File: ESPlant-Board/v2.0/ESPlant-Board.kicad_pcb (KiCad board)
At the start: 2 copper layers, 24 x 181.8 mm, 31 parts, among them J1 Conn_02x04_Counter_Clockwise, U1 ESP32-S2-MINI-1-N4, U2 BH-AAA-B5AK001, U3 Reset, U4 Boot, U5 Temp/Humid-Sensor, U6 Light sensor, U7 AMS1117-3_3, U8 MK-12C02-G025

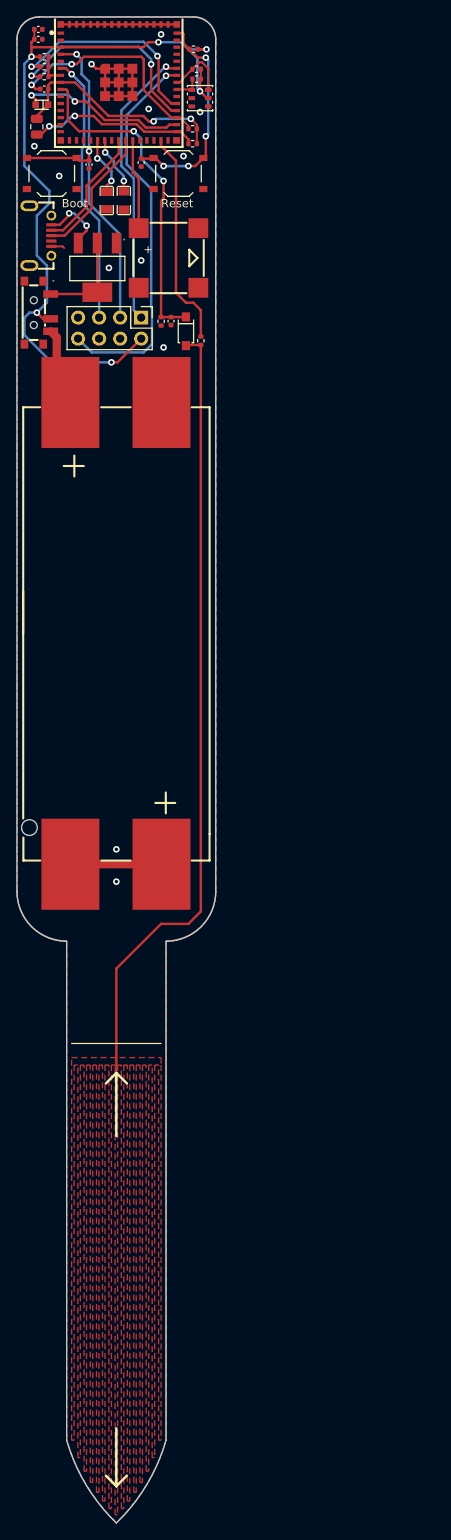
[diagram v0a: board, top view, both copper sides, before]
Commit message: Board: Update panel
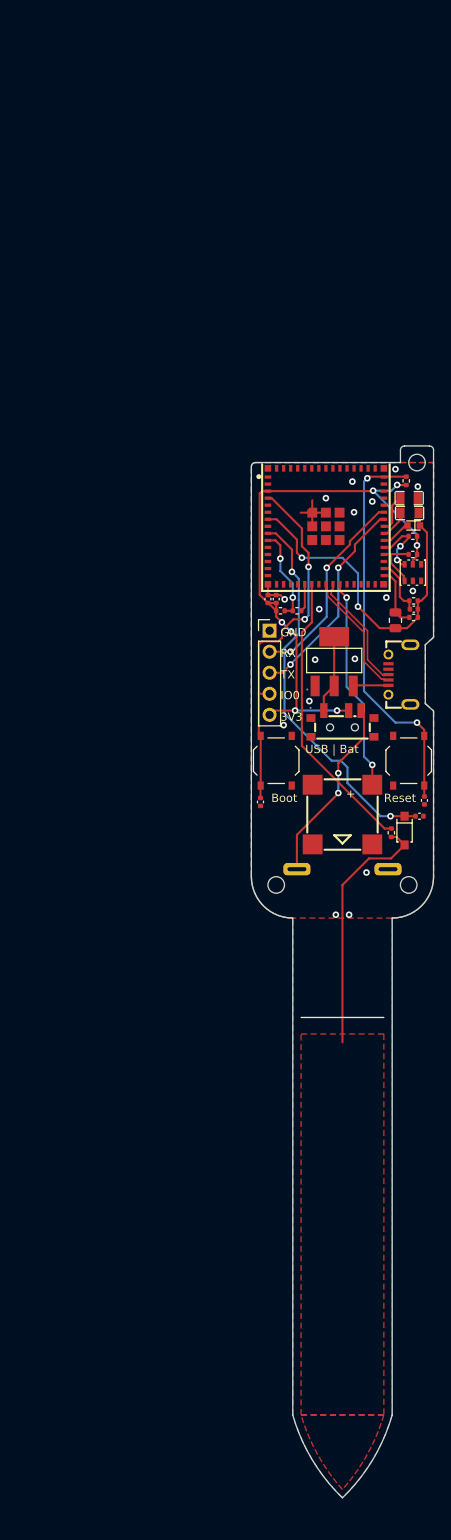
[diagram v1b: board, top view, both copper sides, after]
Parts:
- removed R5: 10k, Resistor_SMD:R_0402_1005Metric
- removed R7: 1M, Resistor_SMD:R_0402_1005Metric
- removed U2: BH-AAA-B5AK001, CustomFootprints:BAT-SMD_BH-AAA-B5AA001
- added U9: ~, CustomFootprints:AAA Battery-spring, B.Cu at (248.5, 149.1)
- C3: value 1uF -> 150pF
- J1: value Conn_02x04_Counter_Clockwise -> Conn_01x05; footprint Connector_PinHeader_2.54mm:PinHeader_2x04_P2.54mm_Vertical -> Connector_PinHeader_2.54mm:PinHeader_1x05_P2.54mm_Vertical
- moved C1 84.3 mm to (258.4, 140.8)
- moved C2 79.7 mm to (238.6, 141.0)
- moved C5 77.0 mm to (257.2, 117.7)
- moved U3 76.2 mm to (256.5, 136.0), turned to 90 degrees
- moved U4 75.9 mm to (240.5, 136.0), turned to -90 degrees
- moved C8 74.5 mm to (240.5, 116.5), turned to 90 degrees
- moved C7 73.7 mm to (254.9, 119.0), turned to 90 degrees
- moved C9 73.0 mm to (239.5, 116.5), turned to 90 degrees
- moved R4 72.7 mm to (241.1, 117.9)
- moved R6 71.4 mm to (243.1, 117.9), turned to 0 degrees
- moved BZ1 70.4 mm to (248.5, 142.5), turned to 180 degrees
- moved USB1 68.5 mm to (255.4, 125.6), turned to 90 degrees
- moved U6 67.8 mm to (257.1, 107.6)
- moved C3 66.9 mm to (257.8, 142.7), turned to 180 degrees
- moved D2 65.8 mm to (256.0, 144.4)
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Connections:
- J1 pad 1: /RX -> GND
- J1 pad 2: +3V3 -> /RX
- J1 pad 3: /IO0 -> /TX
- J1 pad 4: unconnected-(J1-Pin_4-Pad4) -> /IO0
- J1 pad 5: /IO2 -> +3V3
- R6 pad 2: /Voltage_Measurement_Select_2 -> /Voltage_Measurement_Select
- U1 pad 10: unconnected-(U1-IO6-Pad10) -> /Voltage_Measurement_Analog
- U1 pad 20: /LED_GREEN -> /Voltage_Measurement_Select
- U1 pad 21: /LED_RED -> /Square_Wave_Signal
- U1 pad 29: /Square_Wave_Signal -> unconnected-(U1-IO34-Pad29)
- U1 pad 32: /Light_Sensor_In -> /Light_Sensor_Select_1
- U1 pad 33: /Light_Sensor_Select_1 -> unconnected-(U1-IO37-Pad33)
- U1 pad 34: /Voltage_Measurement_Select_2 -> /TH_SDA
- U1 pad 35: /Voltage_Measurement_Select_1 -> /TH_SCL
- U1 pad 36: unconnected-(U1-IO40-Pad36) -> /Light_Sensor_In
- U1 pad 37: /TH_SDA -> /LED_RED
- U1 pad 38: /TH_SCL -> /LED_GREEN
- U1 pad 6: /IO2 -> unconnected-(U1-IO2-Pad6)
- U1 pad 7: /Voltage_Measurement_Analog -> /Light_Sensor_Analog
- U1 pad 8: /Light_Sensor_Analog -> unconnected-(U1-IO4-Pad8)
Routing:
- net /SensorCapV: track 95.6 -> 30.5 mm
- net /IO2: track 32.6 -> 0.00 mm, vias 1 -> 0
- net GND: track 37.3 -> 9.77 mm, vias 12 -> 17
- net /Voltage_Measurement_Select_2: track 25.5 -> 0.00 mm, vias 2 -> 0
- net /Voltage_Measurement_Select_1: track 25.3 -> 0.00 mm, vias 2 -> 0
- net +3V3: track 93.6 -> 70.4 mm, vias 6 -> 7
- net /EN: track 26.2 -> 47.9 mm, vias 4 -> 2
- net /TX: track 47.0 -> 25.4 mm, vias 1 -> 2
- net /Light_Sensor_Select_1: track 27.6 -> 7.01 mm, vias 2 -> 0
- net /Light_Sensor_In: track 20.7 -> 3.60 mm, vias 2 -> 0
- net /Buzzer: track 10.9 -> 25.9 mm, vias 0 -> 2
- net /Light_Sensor_Select_2: track 20.9 -> 7.37 mm, vias 2 -> 0
- net Net-(U9-+): track 9.59 -> 23.1 mm, vias 0 -> 2
- net /Light_Sensor_Analog: track 27.4 -> 39.5 mm
- net Net-(U2-+-Pad3): track 11.0 -> 0.00 mm
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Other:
- board size 24 x 181.8 mm -> 22 x 127 mm
- board text added: "+"
- board text added: "-"
- board text added: "30°"
- board text added: "M2"
- board text removed: "ES-Plant V2.0"
- board text removed: "IO2"
- board text removed: "JLCJLCJLCJLC"
- board text removed: "NC"
